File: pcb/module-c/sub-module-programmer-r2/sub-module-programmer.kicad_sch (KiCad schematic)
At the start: 41 parts, among them J1 Conn_01x06, J2 Conn_01x03, J3 Conn_01x06, J4 Conn_01x06, J5 Conn_01x06, J6 Conn_01x06, J7 Conn_01x06, J8 Serial Bridge, U1 74AHCT1G125, U4 LD1117S33TR_SOT223

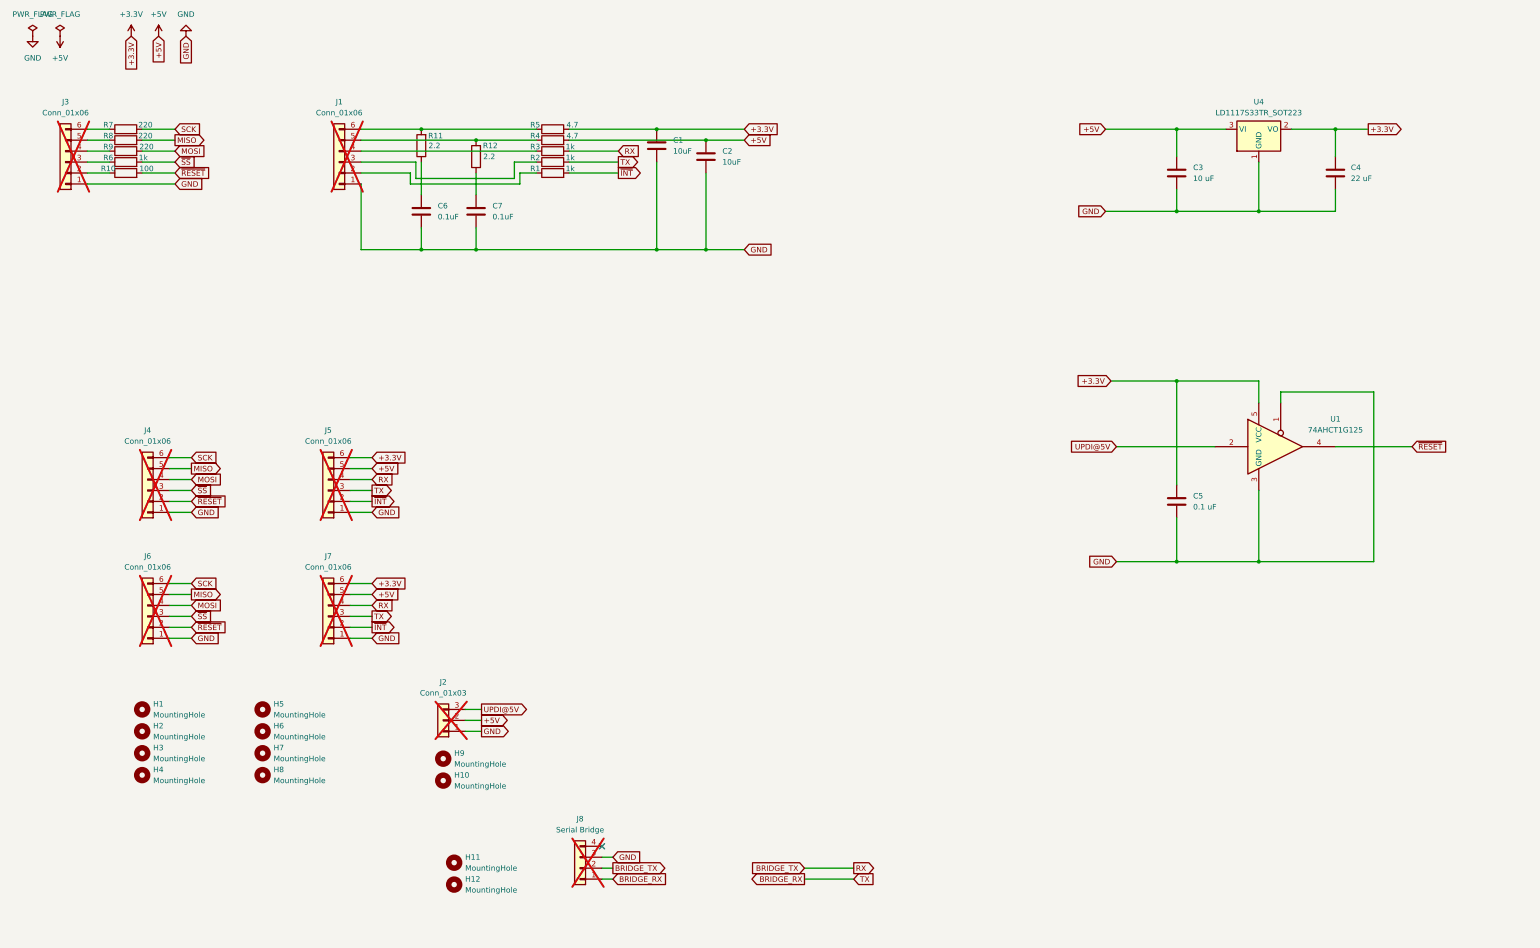
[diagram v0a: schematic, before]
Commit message: Update pcb revisions
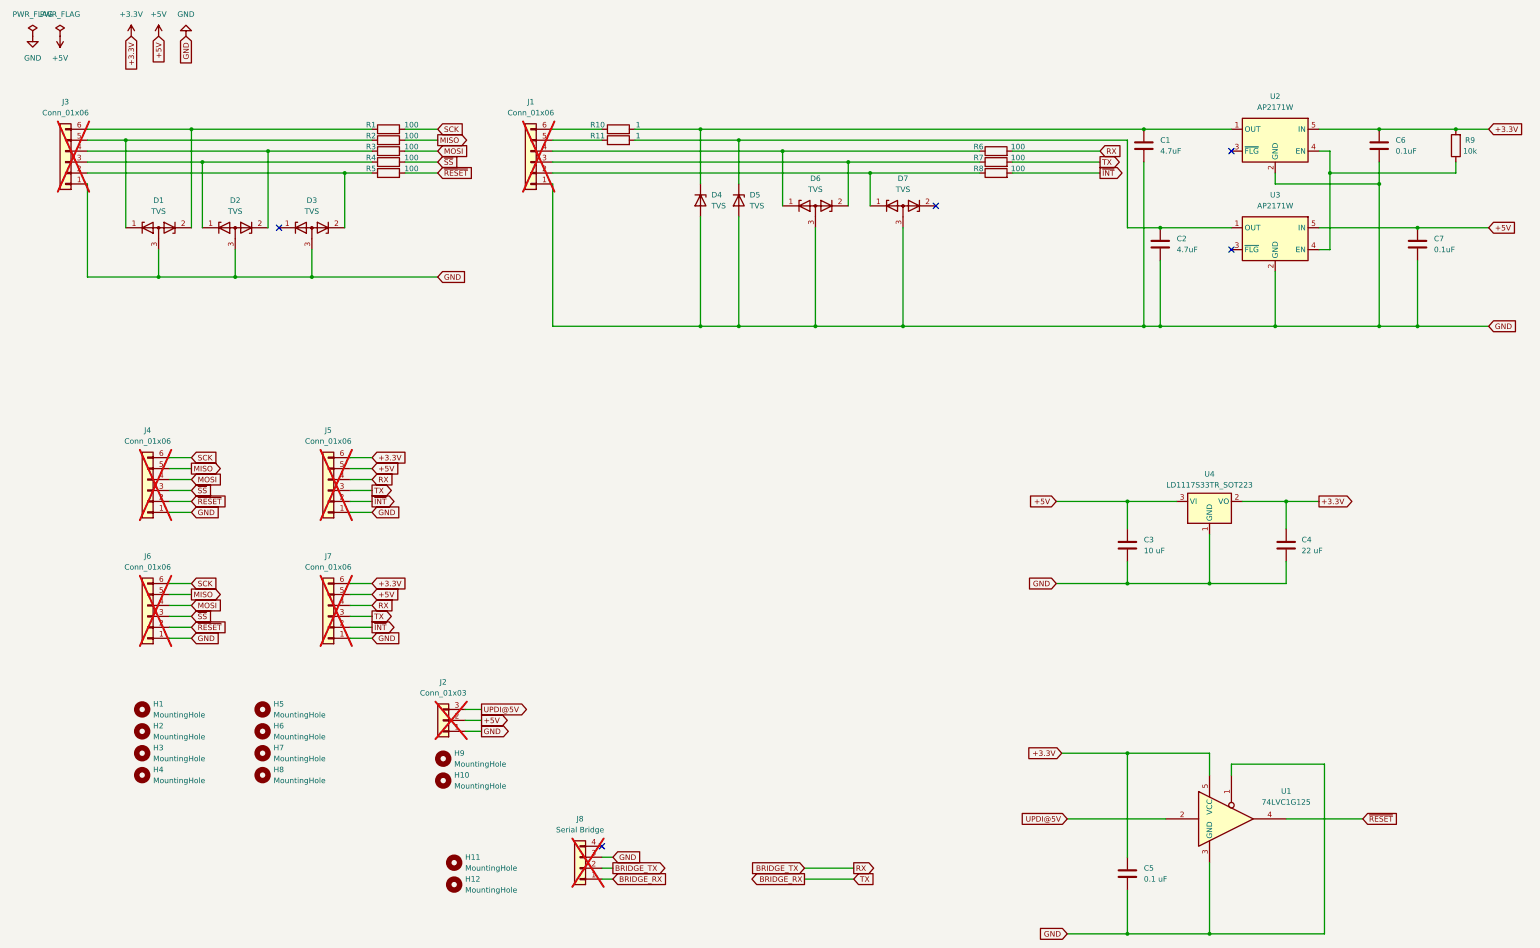
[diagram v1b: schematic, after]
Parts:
- removed R12: 2.2, Resistor_SMD:R_0603_1608Metric, symbol Device:R
- removed R4, R5: 4.7, Resistor_SMD:R_1206_3216Metric, symbol Device:R
- added D1, D2, D3, D6, D7: TVS, Package_TO_SOT_SMD:SOT-723, symbol Device:D_Zener_Dual_CommonAnode_KKA
- added D4, D5: TVS, Diode_SMD:Nexperia_CFP3_SOD-123W, symbol Device:D_Zener
- added R10: 1, Resistor_SMD:R_0805_2012Metric, symbol Device:R
- added R9: 10k, Resistor_SMD:R_0603_1608Metric, symbol Device:R
- added U2, U3: AP2171W, Package_TO_SOT_SMD:SOT-23-5, symbol Power_Management:AP2171W
- C1, C2: value 10uF -> 4.7uF; footprint Capacitor_SMD:C_1206_3216Metric -> Capacitor_SMD:C_0805_2012Metric
- R1: renamed from R7; value 220 -> 100; footprint Resistor_SMD:R_1206_3216Metric -> Resistor_SMD:R_0603_1608Metric
- R11: value 2.2 -> 1; footprint Resistor_SMD:R_0603_1608Metric -> Resistor_SMD:R_0805_2012Metric
- R2: renamed from R8; value 220 -> 100; footprint Resistor_SMD:R_1206_3216Metric -> Resistor_SMD:R_0603_1608Metric
- R3: renamed from R9; value 220 -> 100; footprint Resistor_SMD:R_1206_3216Metric -> Resistor_SMD:R_0603_1608Metric
- R4: renamed from R6; value 1k -> 100; footprint Resistor_SMD:R_1206_3216Metric -> Resistor_SMD:R_0603_1608Metric
- R5: renamed from R10; footprint Resistor_SMD:R_1206_3216Metric -> Resistor_SMD:R_0603_1608Metric
- R6: renamed from R3; value 1k -> 100; footprint Resistor_SMD:R_1206_3216Metric -> Resistor_SMD:R_0603_1608Metric
- R7: renamed from R2; value 1k -> 100; footprint Resistor_SMD:R_1206_3216Metric -> Resistor_SMD:R_0603_1608Metric
- R8: renamed from R1; value 1k -> 100; footprint Resistor_SMD:R_1206_3216Metric -> Resistor_SMD:R_0603_1608Metric
- U1: value 74AHCT1G125 -> 74LVC1G125
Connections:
- net +3.3V: now also C6.1, R9.2, U2.5 (IN); no longer C1.1
- net +5V: now also C7.1, U3.5 (IN); no longer C2.1
- net GND: now also D1.3 (A), D2.3 (A), D3.3 (A), D4.2 (A), D5.2 (A), D6.3 (A), D7.3 (A), U2.2 (GND), U3.2 (GND)
- net at J1.2 (Pin_2), R8.1: now also D7.1 (K)
- net at J1.5 (Pin_5): now also R11.1
- net at J3.2 (Pin_2), R5.1: now also D3.2 (K)
- net at J3.4 (Pin_4), R3.1: now also D2.2 (K)
- net at R11.2: now also C2.1, D5.1 (K), U3.1 (OUT); no longer J1.6 (Pin_6)
- net at J3.3 (Pin_3), R4.1: now also D2.1 (K)
- net at J3.5 (Pin_5), R2.1: now also D1.1 (K)
- net at J3.6 (Pin_6), R1.1: now also D1.2 (K)
- net at J1.3 (Pin_3), R7.1: now also D6.2 (K)
- net at J1.4 (Pin_4), R6.1: now also D6.1 (K)
- new net: C1.1, D4.1 (K), R10.2, U2.1 (OUT)
- new net: R9.1, U2.4 (EN), U3.4 (EN)
- new net: J1.6 (Pin_6), R10.1
- no-connect marks 1 -> 5
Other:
- moved on the sheet: C3, C4, C5, J1, R1, R2, R3, R4, R5, R6, R7, R8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
